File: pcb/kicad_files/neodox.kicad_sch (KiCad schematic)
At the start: 82 parts, among them J1 Conn_01x02_Female, SW1 SW_DPDT_x2, U1 ProMicro

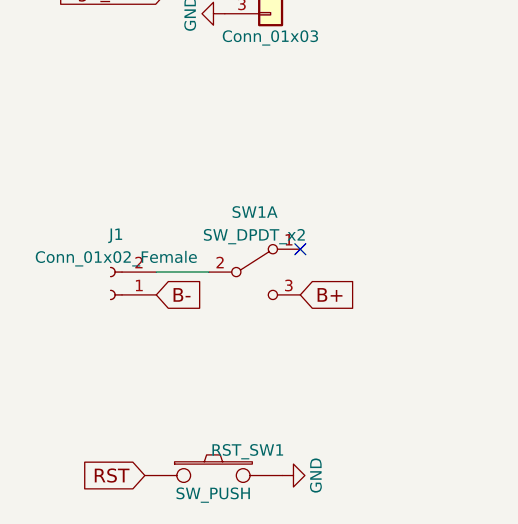
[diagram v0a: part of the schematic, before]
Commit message: Build and pcb changes
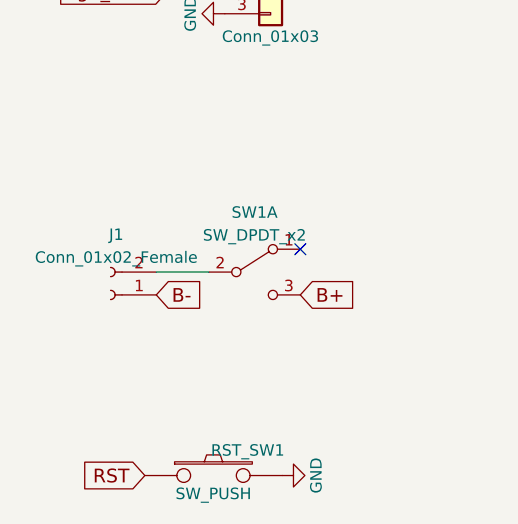
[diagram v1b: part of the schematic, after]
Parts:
- S1, S10, S11, S12, S13, S14, S15, S16, S17, S18, S19, S2, S20, S21, S22, S23, S24, S25, S26, S27, S28, S29, S3, S30, S31, S32, S33, S34, S35, S4, S5, S6, S7, S8, S9: footprint Keyboard_reversible:Kailh_socket_MX_optional_reversible -> keyboard_reversible:Kailh_socket_MX_optional_reversible
